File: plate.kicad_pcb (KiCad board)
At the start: 2 copper layers, 229 x 79.3 mm, 0 parts

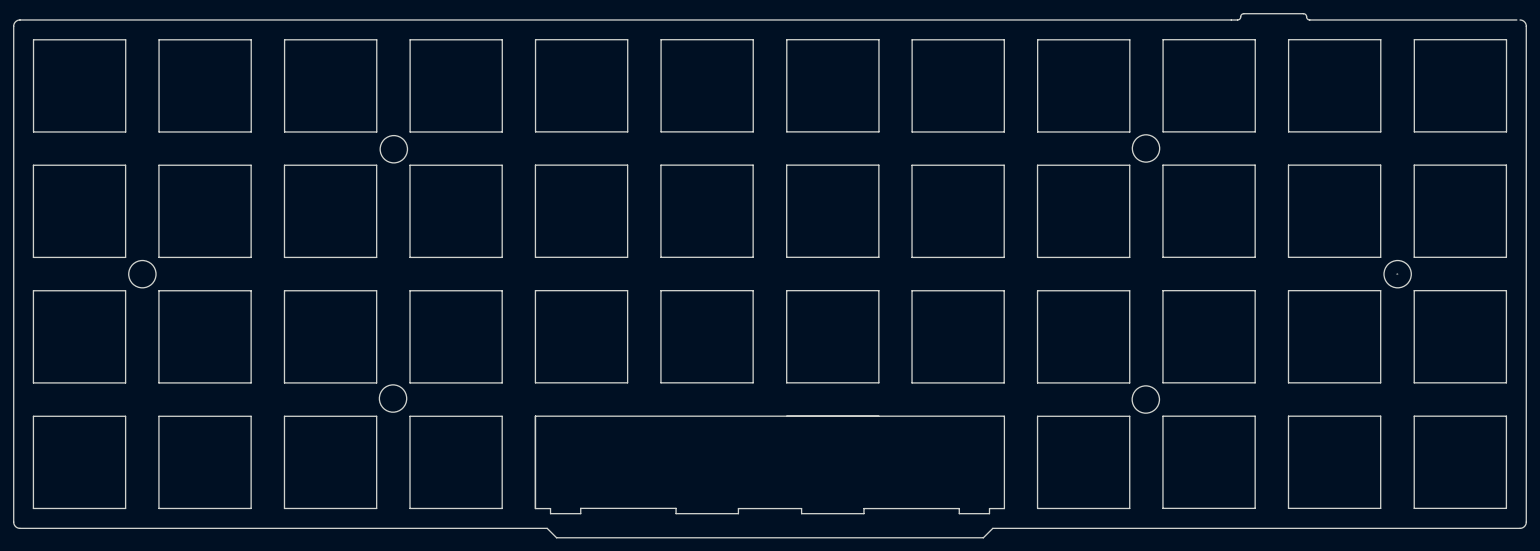
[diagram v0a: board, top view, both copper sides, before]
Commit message: Changed board size for Planck case compatibility
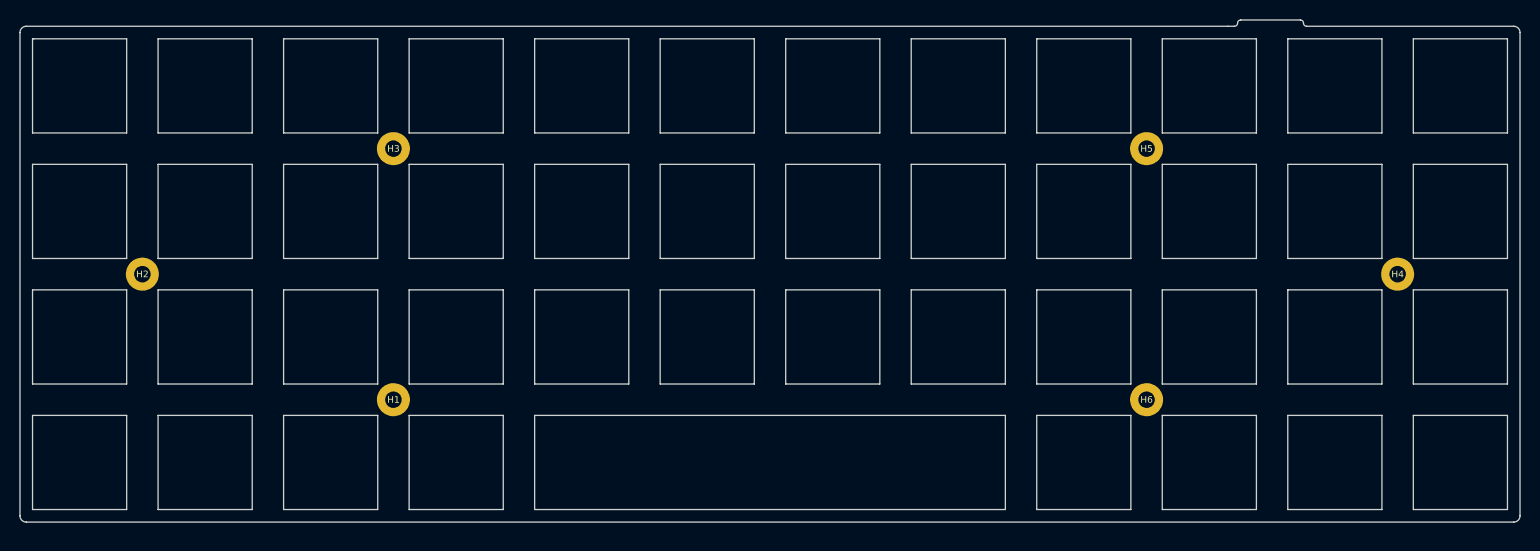
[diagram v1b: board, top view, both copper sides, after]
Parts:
- added H1: MountingHole, MountingHole:MountingHole_2.5mm_Pad, F.Cu at (91.2, 121.6)
- added H2: MountingHole, MountingHole:MountingHole_2.5mm_Pad, F.Cu at (53.2, 102.6)
- added H3: MountingHole, MountingHole:MountingHole_2.5mm_Pad, F.Cu at (91.2, 83.6)
- added H4: MountingHole, MountingHole:MountingHole_2.5mm_Pad, F.Cu at (243.2, 102.6)
- added H5: MountingHole, MountingHole:MountingHole_2.5mm_Pad, F.Cu at (205.2, 83.6)
- added H6: MountingHole, MountingHole:MountingHole_2.5mm_Pad, F.Cu at (205.2, 121.6)
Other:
- board size 229 x 79.3 mm -> 227.1 x 76 mm
